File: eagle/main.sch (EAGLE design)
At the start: 36 parts, among them Q1 SQJ886EP, U1 LTC3789EGNPBF

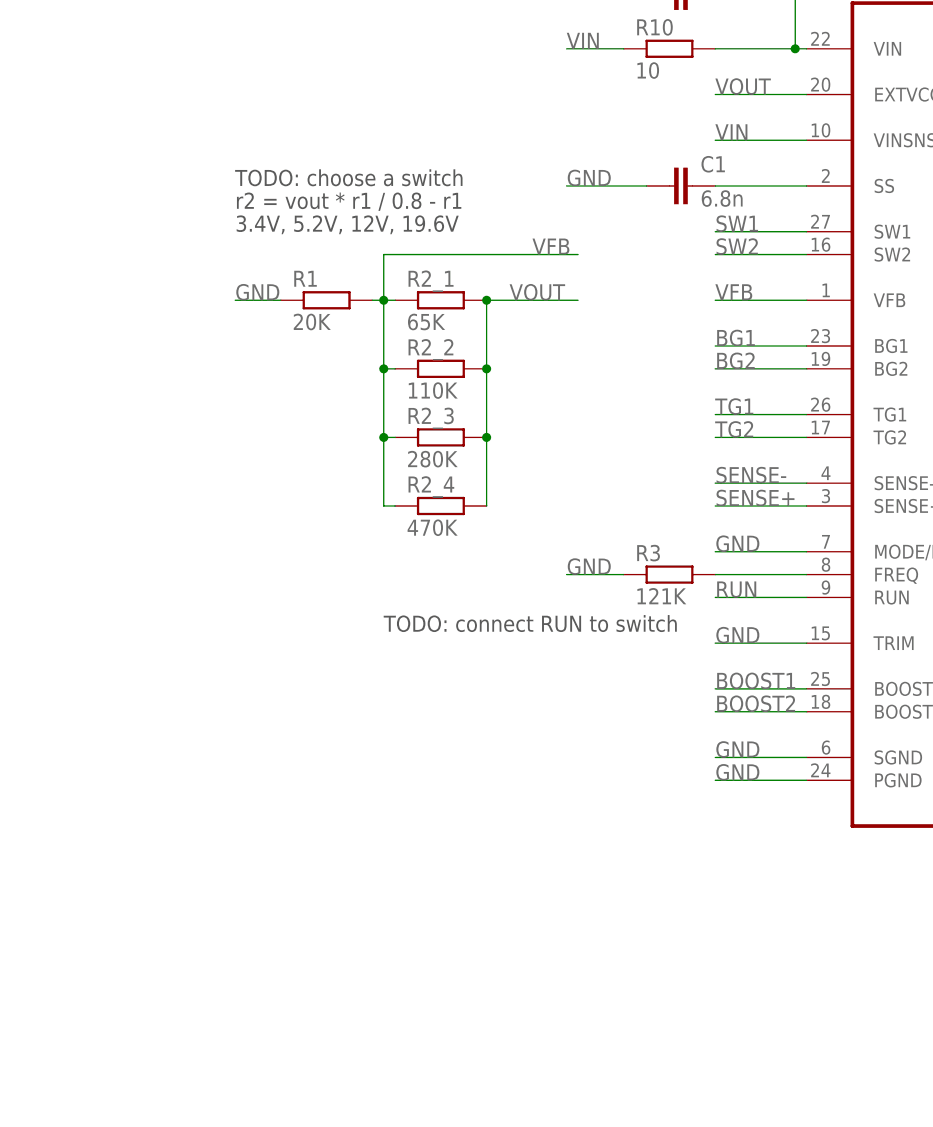
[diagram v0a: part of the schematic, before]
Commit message: [ update ] sch
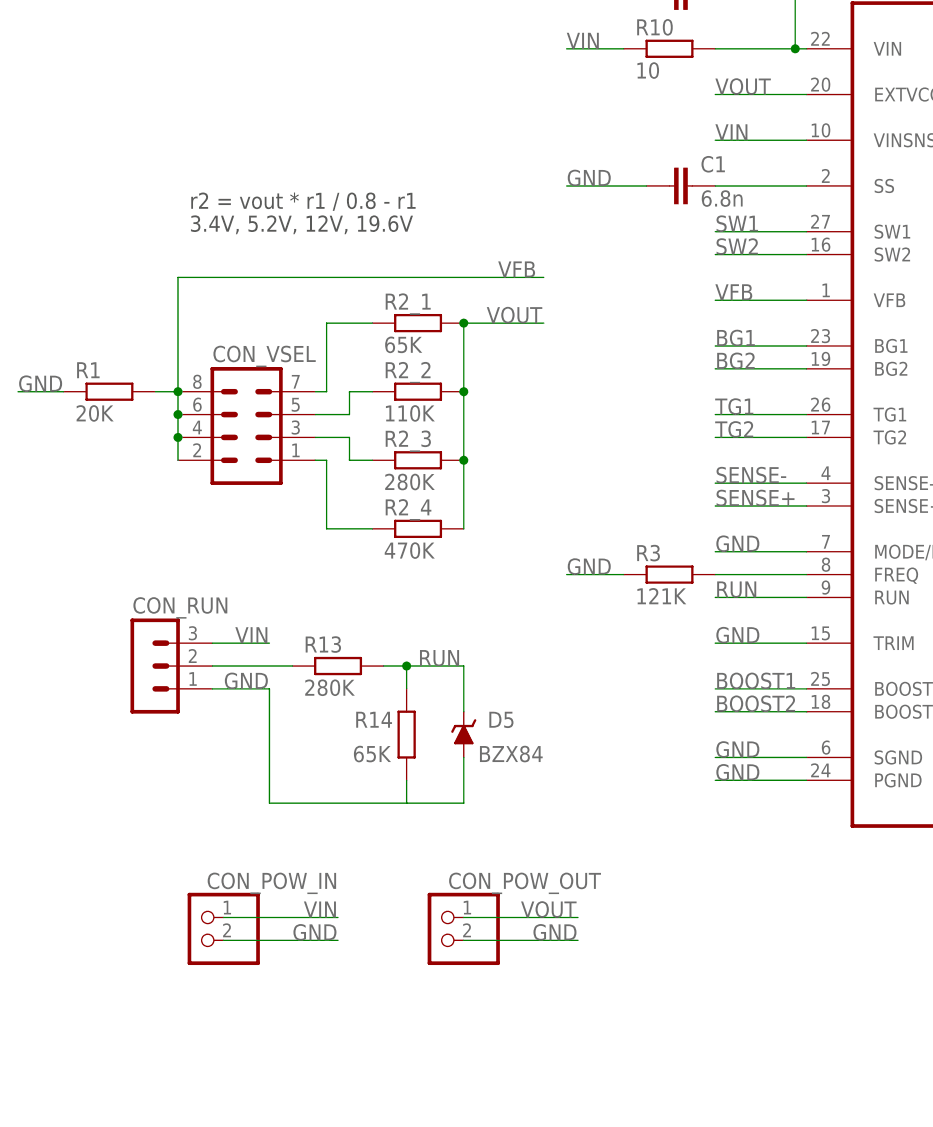
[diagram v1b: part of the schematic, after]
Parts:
- added CON_POW_IN, CON_POW_OUT: (no value), pinhead:PINHD-1X2
- added CON_RUN: (no value), con-lstb:MA03-1
- added CON_VSEL: (no value), con-lstb:MA04-2
- added D5: BZX84, diode:BZX84
- added R13: 280K, resistor:R-EU_R1206
- added R14: 65K, resistor:R-EU_R1206
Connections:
- new net N$10: CON_VSEL.3, R2_3.1
- new net N$11: CON_RUN.2, R13.1
- new net N$7: CON_VSEL.5, R2_2.1
- new net N$8: CON_VSEL.7, R2_1.1
- net GND: now also CON_POW_IN.2, CON_POW_OUT.2, CON_RUN.1, D5.A, R14.1
- net RUN: now also D5.C, R13.2, R14.2
- net VFB: now also CON_VSEL.1, CON_VSEL.2, CON_VSEL.4, CON_VSEL.6, CON_VSEL.8; no longer R2_1.1, R2_2.1, R2_3.1
- net VIN: now also CON_POW_IN.1, CON_RUN.3
- net VOUT: now also CON_POW_OUT.1
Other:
- note removed: "TODO: choose a switch"
- note removed: "TODO: connect RUN to switch"
- moved on the sheet: R1, R2_1, R2_2, R2_3, R2_4
